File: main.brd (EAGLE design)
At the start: 50 x 95 mm, 213 parts, among them CN1 USB C 2.0, CN2 JST GH 10 Pin, CN3 15PIN 0.5MM, CN4 8 PIN FFC, CN5 NEB-21-R, CN6 S4B-XH-SM4-TB, CN7 8 PIN FFC, Q1 GSFP0449, Q2 2SCR586D, Q3 MMBT3904, SW1 DPDT, U1 TPS54302, U10 SN74LVC2G17, U11 SN74LVC2G17, U12 SN74LVC2G17, U13 SN74LVC2G17, U14 SN74LVC2G17, U15 SN74LVC2G17, U16 SN74LVC2G17, U17 SN74LVC2G17, U18 T8Q144C4, U19 SN74LVC2G17, U2 USBLC6-2SC6, U20 R2A20169SA#W5, U21 LM317MDT, U22 LM317MDT, U23 TMC2208-LA-T, U3 93LC56B-I/SN, U33 LM317MDT, U34 LM317MDT, U4 W25Q128JV, U5 TPS62065, U6 FT2232H, U7 TPS563201, U8 TCD2720BFG, U9 SN74LVC2G17

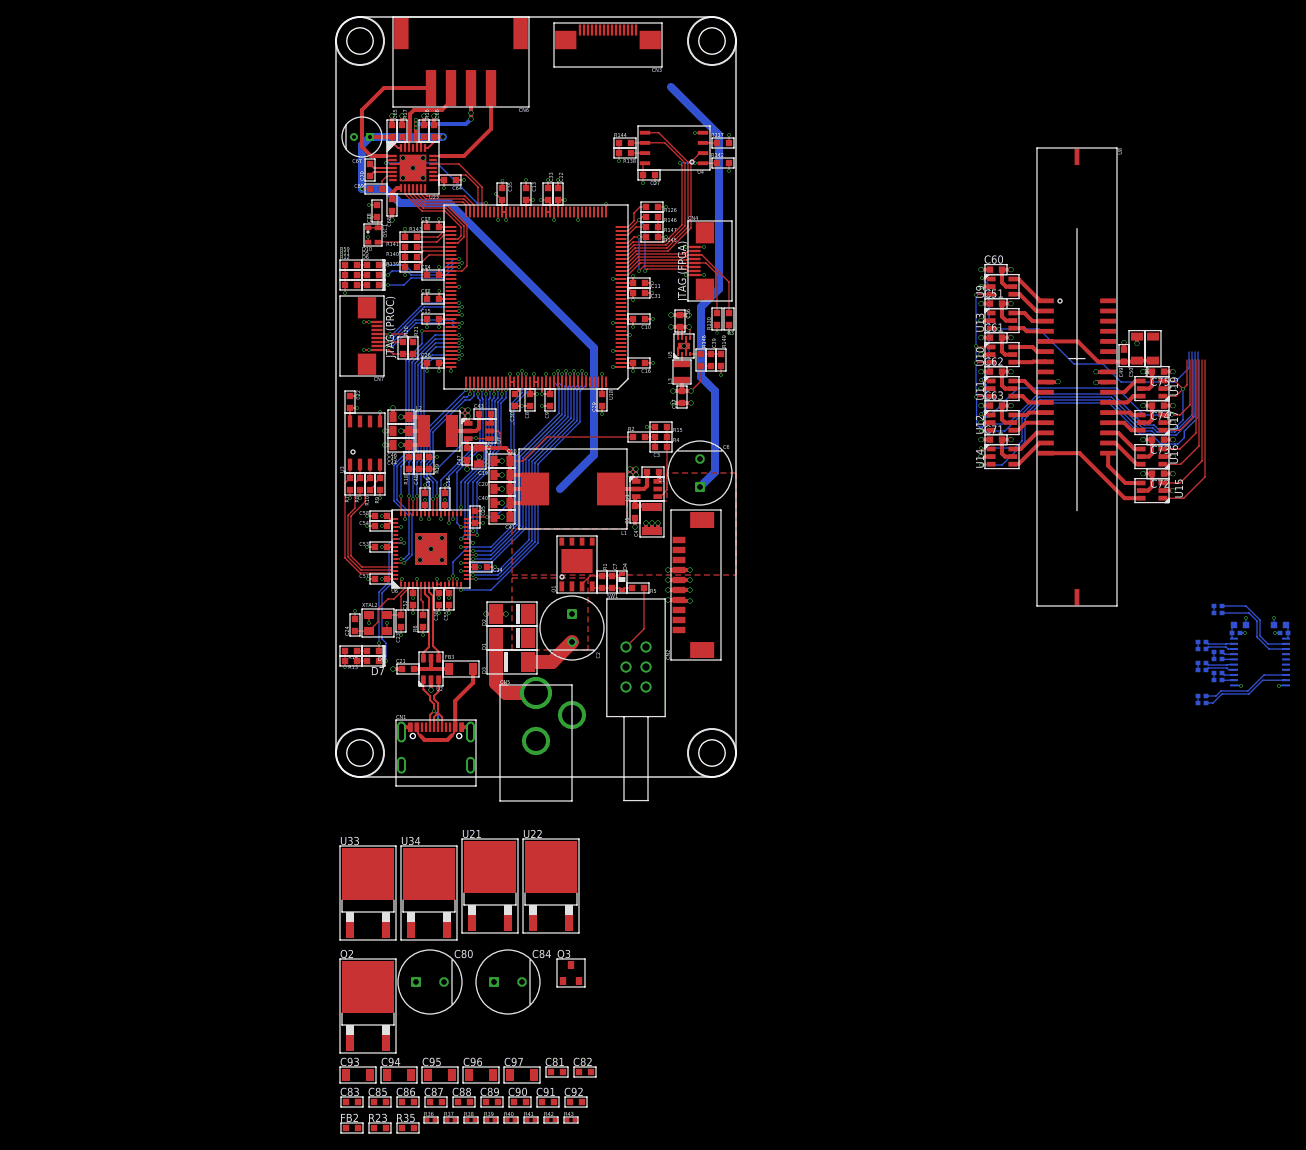
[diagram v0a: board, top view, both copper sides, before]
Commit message: FTDI and CCD routed
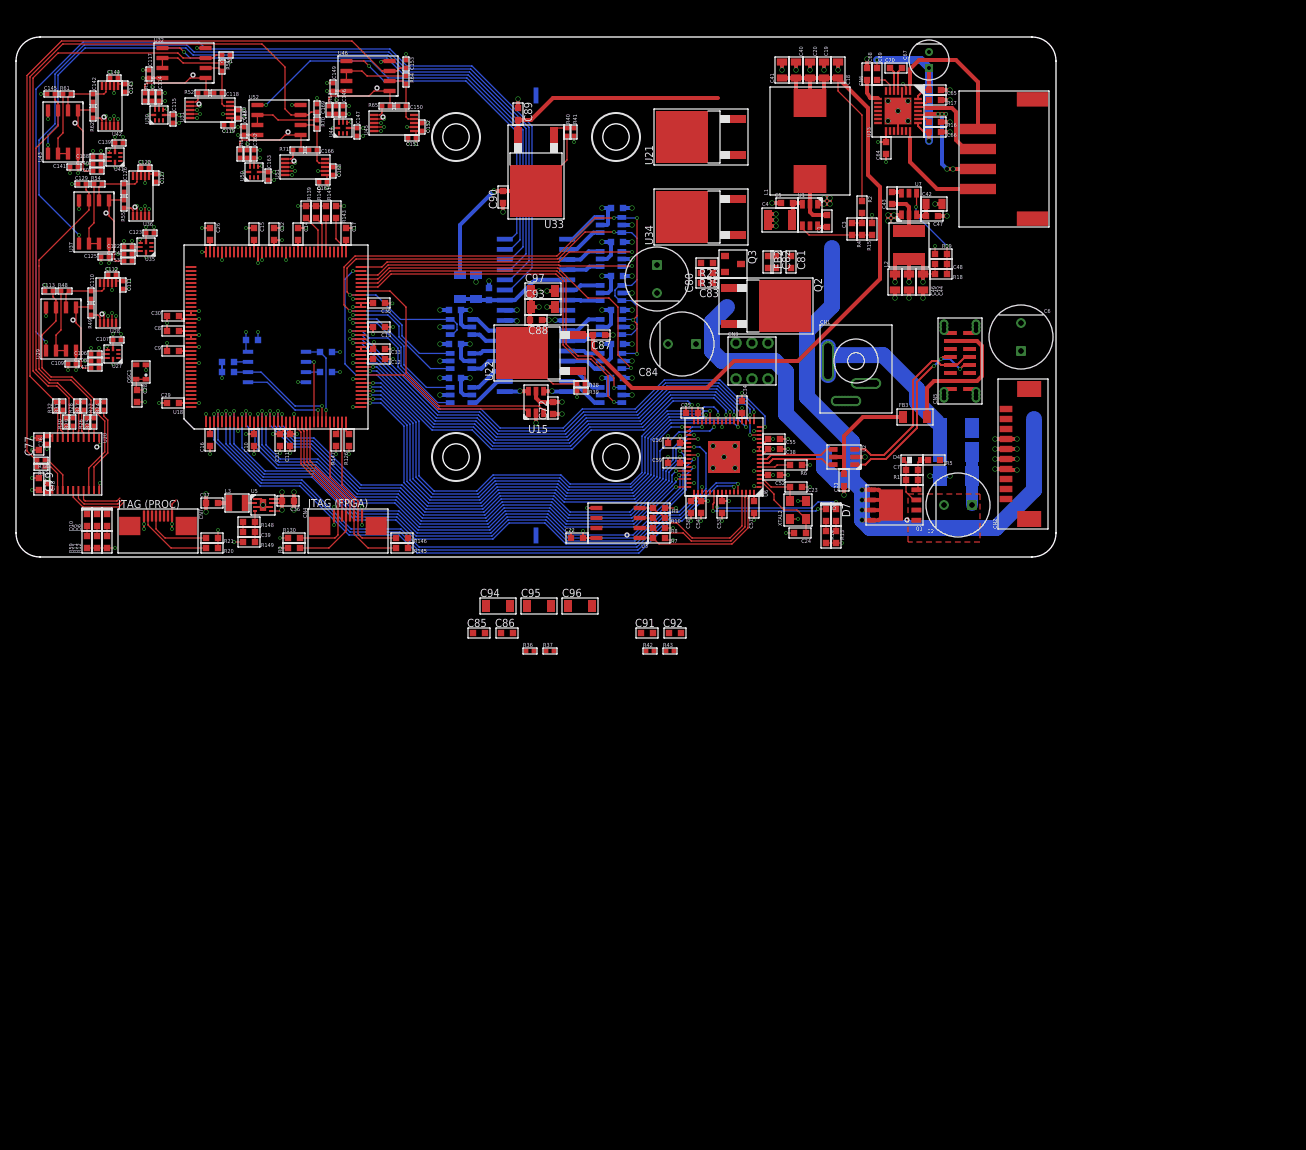
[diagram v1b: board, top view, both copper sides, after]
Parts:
- removed SW1: DPDT, ELECTROMECH:PBH2UEESNPNAGX
- added C106, C107, C109, C111, C112, C113, C114, C115, C117, C119, C120, C121, C122, C123, C125, C127, C128, C129, C138, C139, C141, C143, C144, C145, C146, C147, C149, C151, C152, C153, C162, C163, C165, C167, C168, C169: 0.1uF 16V, c_0402:0402
- added C108, C116, C124, C140, C148, C164: 220pF 25V, c_0402:0402
- added C110, C118, C126, C142, C150, C166: NO FIT, c_0402:0402
- added R47, R50, R53, R60, R63, R69: 100R, r_0402:0402
- added R48, R51, R54, R61, R64, R70: 330R, r_0402:0402
- added R49, R52, R55, R62, R65, R71: 680R, r_0402:0402
- added U27, U30, U35, U41, U44, U50: ADS7056, ICs:X2QFN8
- added U28, U31, U36, U42, U45, U51: AD5258BRMZ1-R7, ICs:MSOP10
- added U29, U32, U37, U43, U46, U52: COS8092SR, ICs:SO8
- CN1: value USB C 2.0 -> DC-012A-D010; device CONNECTORs:MC-107D -> CONNECTORs:DC-012A-D010
- CN3: value 15PIN 0.5MM -> 5.8ZSPT; device CONNECTORs:SFV15R-1STE1HLF -> ELECTROMECH:5.8ZSPT
- CN5: value NEB-21-R -> MC-118LS-H100; device CONNECTORs:NEB-21-R -> CONNECTORs:MC-118LS-H100
- R41: value 715R -> 1.69k
- R43: value 715R -> 390R
- moved C79 156.1 mm to (-62.1, -23.4), flipped to the top, turned to 270 degrees
- moved C78 155.7 mm to (-61.1, -23.9), flipped to the top, turned to 270 degrees
- moved C77 151.8 mm to (-62.1, -18.4), flipped to the top, turned to 90 degrees
- moved C76 150.6 mm to (-61.1, -17.9), flipped to the top, turned to 90 degrees
- moved U20 150.1 mm to (-57.5, -20.9), flipped to the top, turned to 270 degrees
- moved R34 148.4 mm to (-61.9, -20.4), flipped to the top, turned to 180 degrees
- moved R33 148.1 mm to (-61.9, -21.3), flipped to the top, turned to 180 degrees
- moved R30 146.9 mm to (-58.8, -15.6), flipped to the top, turned to 90 degrees
- moved R32 146.3 mm to (-60.0, -13.6), flipped to the top, turned to 90 degrees
- moved R29 146.2 mm to (-57.9, -15.6), flipped to the top, turned to 90 degrees
- moved R31 145.6 mm to (-59.1, -13.6), flipped to the top, turned to 90 degrees
- moved R26 144.8 mm to (-56.1, -15.6), flipped to the top, turned to 90 degrees
- moved R28 144.3 mm to (-57.4, -13.6), flipped to the top, turned to 90 degrees
- moved R25 144.2 mm to (-55.3, -15.6), flipped to the top, turned to 90 degrees
- moved R27 143.6 mm to (-56.5, -13.6), flipped to the top, turned to 90 degrees
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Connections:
- removed net GPIOB_N0: U18.56
- removed net GPIOB_N2: U18.59
- removed net GPIOB_N3: U18.60
- removed net GPIOB_N7: U18.65
- removed net GPIOB_P0: U18.55
- removed net GPIOB_P2: U18.58
- removed net GPIOB_P3: U18.61
- removed net GPIOB_P7: U18.66
- removed net GPIOB_TN0: U18.39
- removed net GPIOB_TN11: U18.54
- removed net GPIOB_TN2: U18.41
- removed net GPIOB_TN4: U18.43
- removed net GPIOB_TN6: U18.46
- removed net GPIOB_TN9: U18.48
- removed net GPIOB_TP0: U18.38
- removed net GPIOB_TP11: U18.53
- removed net GPIOB_TP2: U18.40
- removed net GPIOB_TP4: U18.42
- removed net GPIOB_TP6: U18.45
- removed net GPIOB_TP9: U18.47
- removed net GPIOL_12: U18.20
- removed net GPIOL_13: U18.19
- removed net GPIOL_20: U18.18
- removed net GPIOL_21: U18.17
- removed net GPIOL_22: U18.16
- removed net GPIOL_24: U18.15
- removed net GPIOL_25: U18.14
- removed net GPIOL_31: U18.11
- removed net GPIOL_32: U18.10
- removed net GPIOL_40: U18.8
- removed net GPIOL_41: U18.7
- removed net GPIOL_46: U18.6
- removed net GPIOL_53: U18.3
- removed net GPIOL_54: U18.4
- removed net PWR_LED_24V: C4.2, C5.2, C6.P, CN2.10, CN2.8, CN2.9, Q1.5, Q1.6, Q1.7, Q1.8, Q1.PAD, U1.3
- new net ADC_SPI_MISO_1: U27.2
- new net ADC_SPI_MISO_2: U35.2
- new net ADC_SPI_MISO_3: U41.2
- new net ADC_SPI_MISO_4: U30.2
- new net ADC_SPI_MISO_5: U44.2
- new net ADC_SPI_MISO_6: U50.2
- new net ADC_SPI_NCS: U27.1, U30.1, U35.1, U41.1, U44.1, U50.1
- new net ADC_SPI_SCLK: U27.3, U30.3, U35.3, U41.3, U44.3, U50.3
- new net N$100: R70.1, U52.6, U52.7
- new net N$61: C108.2, R47.2, U27.7
- new net N$62: C110.2, R47.1, R49.2, U29.1
- new net N$63: C110.1, R48.2, U28.9, U29.2
- new net N$64: R49.1, U28.1
- new net N$65: R48.1, U29.6, U29.7
- new net N$66: C116.2, R50.2, U30.7
- new net N$67: C118.2, R50.1, R52.2, U32.1
- new net N$68: C118.1, R51.2, U31.9, U32.2
- new net N$69: R52.1, U31.1
- new net N$70: R51.1, U32.6, U32.7
- new net N$71: C124.2, R53.2, U35.7
- new net N$72: C126.2, R53.1, R55.2, U37.1
- new net N$73: C126.1, R54.2, U36.9, U37.2
- new net N$74: R55.1, U36.1
- new net N$75: R54.1, U37.6, U37.7
- new net N$81: C140.2, R60.2, U41.7
- new net N$82: C142.2, R60.1, R62.2, U43.1
- new net N$83: C142.1, R61.2, U42.9, U43.2
- new net N$84: R62.1, U42.1
- new net N$85: R61.1, U43.6, U43.7
- new net N$86: C148.2, R63.2, U44.7
- new net N$87: C150.2, R63.1, R65.2, U46.1
- new net N$88: C150.1, R64.2, U45.9, U46.2
- new net N$89: R65.1, U45.1
- new net N$90: R64.1, U46.6, U46.7
- new net N$96: C164.2, R69.2, U50.7
- new net N$97: C166.2, R69.1, R71.2, U52.1
- new net N$98: C166.1, R70.2, U51.9, U52.2
- new net N$99: R71.1, U51.1
- new net POT_I2C0_SCL: U28.5, U36.5, U42.5
- new net POT_I2C0_SDA: U28.4, U36.4, U42.4
- new net POT_I2C1_SCL: U31.5, U45.5, U51.5
- new net POT_I2C1_SDA: U31.4, U45.4, U51.4
- net CCD_SH_M1: now also U15.4; no longer U15.6
- net CCD_SH_M2: now also U15.6; no longer U15.4
- net CCD_SIG_1A: now also U18.61
- net CCD_SIG_2A: now also U18.65
- net CCD_SIG_CP: now also U18.72
- net CCD_SIG_RS: now also U18.70
- net CCD_SIG_SH_M1: now also U15.3, U18.66; no longer U15.1
- net CCD_SIG_SH_M2: now also U15.1, U18.45; no longer U15.3
- net CCD_SIG_SH_S1: now also U18.67
- net CCD_SIG_SH_S2: now also U18.58
- net CCD_SIG_SH_S3: now also U18.68
- net CCD_SIG_SH_S4: now also U18.59
- net CCD_SIG_SW: now also U18.60
- net CCD_SIG_TG: now also U18.69
- net FPGA_CONF_CSI: now also CN4.3; no longer CN4.6
- net FPGA_CONF_NCRST: now also CN4.2; no longer CN4.7
- net FPGA_JTAG_TCK: now also CN4.5; no longer CN4.3
- net FPGA_JTAG_TDI: now also CN4.4; no longer CN4.2
- net FPGA_JTAG_TDO: now also CN4.7; no longer CN4.5
- net FPGA_JTAG_TMS: now also CN4.6; no longer CN4.4
- net FPGA_STATUS: no longer U18.83
- net FT_CLKOUT: now also U18.71; no longer U18.123
- net FT_CONT_NCTS: now also U18.10; no longer U18.109
- net FT_CONT_NDCD: now also U18.11; no longer U18.103
- net FT_CONT_NDSR: now also U18.16; no longer U18.105
- net FT_CONT_NDTR: now also U18.8; no longer U18.106
- net FT_CONT_NRI: now also U18.15; no longer U18.102
- net FT_CONT_NRTS: now also U18.7; no longer U18.110
- net FT_CONT_PWRSAV: now also U18.3; no longer U18.99
- net FT_CONT_RX: now also U18.17; no longer U18.111
- net FT_CONT_TX: now also U18.6; no longer U18.112
- net FT_CONT_TXDEN: now also U18.14; no longer U18.101
- net FT_D0: now also U18.56; no longer U18.139
- net FT_D1: now also U18.55; no longer U18.138
- net FT_D2: now also U18.54; no longer U18.137
- net FT_D3: now also U18.40; no longer U18.136
- net FT_D4: now also U18.39; no longer U18.135
- net FT_D5: now also U18.48; no longer U18.134
- net FT_D6: now also U18.47; no longer U18.132
- net FT_D7: now also U18.46; no longer U18.131
- net FT_NOE: now also U18.38; no longer U18.115
- net FT_NPWREN: now also U18.4; no longer U18.100
- net FT_NRD: now also U18.42; no longer U18.119
- net FT_NRST: now also U18.53; no longer U18.124
- net FT_NRXF: now also U18.43; no longer U18.117
- net FT_NSIWU: now also U18.20; no longer U18.114
- net FT_NSUSPEND: now also U18.18; no longer U18.113
- net FT_NTXE: now also U18.19; no longer U18.116
- net FT_NWR: now also U18.41; no longer U18.118
- net GND: now also C106.1, C107.1, C108.1, C109.1, C111.1, C112.1, C113.1, C114.1, C115.1, C116.1, C117.1, C119.1, C120.1, C121.1, C122.1, C123.1, C124.1, C125.1, C127.1, C128.1, C129.1, C138.1, C139.1, C140.1, C141.1, C143.1, C144.1, C145.1, C146.1, C147.1, C148.1, C149.1, C151.1, C152.1, C153.1, C162.1, C163.1, C164.1, C165.1, C167.1, C168.1, C169.1, CN1.-1, CN1.-2, CN1.-3, CN1.-4, CN1.-5, CN1.-6, CN1.-7, CN1.-8, CN3.2, CN5.A1, CN5.A12, CN5.B1, CN5.B12, CN5.SHELL1, CN5.SHELL10, CN5.SHELL11, CN5.SHELL12, CN5.SHELL2, CN5.SHELL3, CN5.SHELL4, CN5.SHELL5, CN5.SHELL6, CN5.SHELL7, CN5.SHELL8, CN5.SHELL9, U27.5, U27.8, U28.2, U28.3, U28.7, U29.4, U30.5, U30.8, U31.2, U31.3, U31.7, U32.4, U35.5, U35.8, U36.3, U36.7, U37.4, U41.5, U41.8, U42.2, U42.7, U43.4, U44.5, U44.8, U45.3, U45.7, U46.4, U50.5, U50.8, U51.2, U51.7, U52.4; no longer CN1.A12B1, CN1.B12A1, CN1.P$1, CN1.P$10, CN1.P$11, CN1.P$12, CN1.P$13, CN1.P$14, CN1.P$15, CN1.P$16, CN1.P$17, CN1.P$18, CN1.P$19, CN1.P$2, CN1.P$20, CN1.P$21, CN1.P$22, CN1.P$23, CN1.P$24, CN1.P$3, CN1.P$4, CN1.P$5, CN1.P$6, CN1.P$7, CN1.P$8, CN1.P$9, CN5.3, SW1.2
- net N$11: now also CN3.3; no longer SW1.3
- net N$12: now also CN5.A6, CN5.B6; no longer CN1.A6, CN1.B6
- net N$13: now also CN5.A7, CN5.B7; no longer CN1.A7, CN1.B7
- net N$41: now also CN5.A4, CN5.A9, CN5.B4, CN5.B9; no longer CN1.A9B4, CN1.B9A4
- net N$5: now also CN1.+1, CN1.+10, CN1.+11, CN1.+2, CN1.+3, CN1.+4, CN1.+5, CN1.+6, CN1.+7, CN1.+8, CN1.+9; no longer CN5.1
- net PROC_JTAG_TCK: now also CN7.5, R21.1; no longer CN7.3, R20.1, U18.97
- net PROC_JTAG_TDI: now also CN7.4; no longer CN7.2, U18.98
- net PROC_JTAG_TDO: now also CN7.7, R20.1; no longer CN7.5, R21.1, U18.92
- net PROC_JTAG_TMS: now also CN7.6; no longer CN7.4, U18.93
- net PROC_SCANNING: no longer U18.81
- net PROC_STATUS: no longer U18.82
- net PWR_ANA_3V3: now also C106.2, C114.2, C122.2, C138.2, C146.2, C162.2, U27.6, U30.6, U35.6, U41.6, U44.6, U50.6
- net PWR_ANA_5V: now also C109.2, C112.2, C117.2, C120.2, C125.2, C128.2, C141.2, C144.2, C149.2, C152.2, C165.2, C168.2, U28.8, U29.8, U31.8, U32.8, U36.8, U37.8, U42.8, U43.8, U45.8, U46.8, U51.8, U52.8
- net PWR_BUS_24V_UNREG: now also C4.2, C5.2, C6.P, CN2.10, CN2.8, CN2.9, Q1.5, Q1.6, Q1.7, Q1.8, Q1.PAD, U1.3
- net PWR_SYS_3V3: now also C107.2, C111.2, C115.2, C119.2, C123.2, C127.2, C139.2, C143.2, C147.2, C151.2, C163.2, C167.2, U27.4, U28.6, U30.4, U31.6, U35.4, U36.2, U36.6, U41.4, U42.3, U42.6, U44.4, U45.2, U45.6, U50.4, U51.3, U51.6
- net SEN_OFFSET_OS1: now also C113.2, U29.3
- net SEN_OFFSET_OS2: now also C129.2, U37.3
- net SEN_OFFSET_OS3: now also C145.2, U43.3
- net SEN_OFFSET_OS4: now also C121.2, U32.3
- net SEN_OFFSET_OS5: now also C153.2, R33.2, R34.2, U46.3; no longer R31.2, R32.2
- net SEN_OFFSET_OS6: now also C169.2, R31.2, R32.2, U52.3; no longer R33.2, R34.2
- net SEN_SIG_OS1: now also U29.5
- net SEN_SIG_OS2: now also U37.5
- net SEN_SIG_OS3: now also U43.5
- net SEN_SIG_OS4: now also U32.5
- net SEN_SIG_OS5: now also U46.5
- net SEN_SIG_OS6: now also U52.5
- net STP_CLK: no longer U18.71
- net STP_DIA: no longer U18.84
- net STP_DIR: no longer U18.68
- net STP_IDX: no longer U18.72
- net STP_MS1: no longer U18.76
- net STP_MS2: no longer U18.77
- net STP_NEN: no longer U18.67
- net STP_STP: no longer U18.69
- net STP_UART_IO: no longer U18.70
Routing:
- net PWR_BUS_24V_UNREG: track 0.00 -> 127.0 mm, vias 0 -> 4
- net SEN_SIG_OS1: track 0.70 -> 125.0 mm, vias 0 -> 1
- net PWR_FPGA_1V2: track 145.9 -> 21.9 mm, vias 13 -> 3
- net SEN_SIG_OS2: track 0.75 -> 110.6 mm, vias 0 -> 1
- net SEN_OFFSET_OS5: track 0.88 -> 100.4 mm
- net SEN_SIG_OS3: track 0.62 -> 94.2 mm, vias 0 -> 1
- net SEN_OFFSET_OS6: track 0.88 -> 87.3 mm
- net SEN_OFFSET_OS4: track 0.88 -> 71.2 mm
- net SEN_SIG_OS4: track 0.00 -> 66.9 mm, vias 0 -> 1
- net FT_CONT_TX: track 19.9 -> 80.8 mm
- net GND: track 170.8 -> 231.4 mm, vias 155 -> 237
- net FT_CONT_NRTS: track 19.2 -> 78.6 mm
- net PWR_LED_24V: track 58.3 -> 0.00 mm
- net SEN_SIG_OS6: track 0.00 -> 54.7 mm, vias 0 -> 1
- net FT_CONT_NCTS: track 20.2 -> 74.2 mm
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- added copper zone on layer 3, net PWR_CLK_5V
- removed copper zone on layer 1, net PWR_LED_24V
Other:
- board size 50 x 95 mm -> 130 x 65 mm

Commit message: Board routed, needs motor driver and thorough review
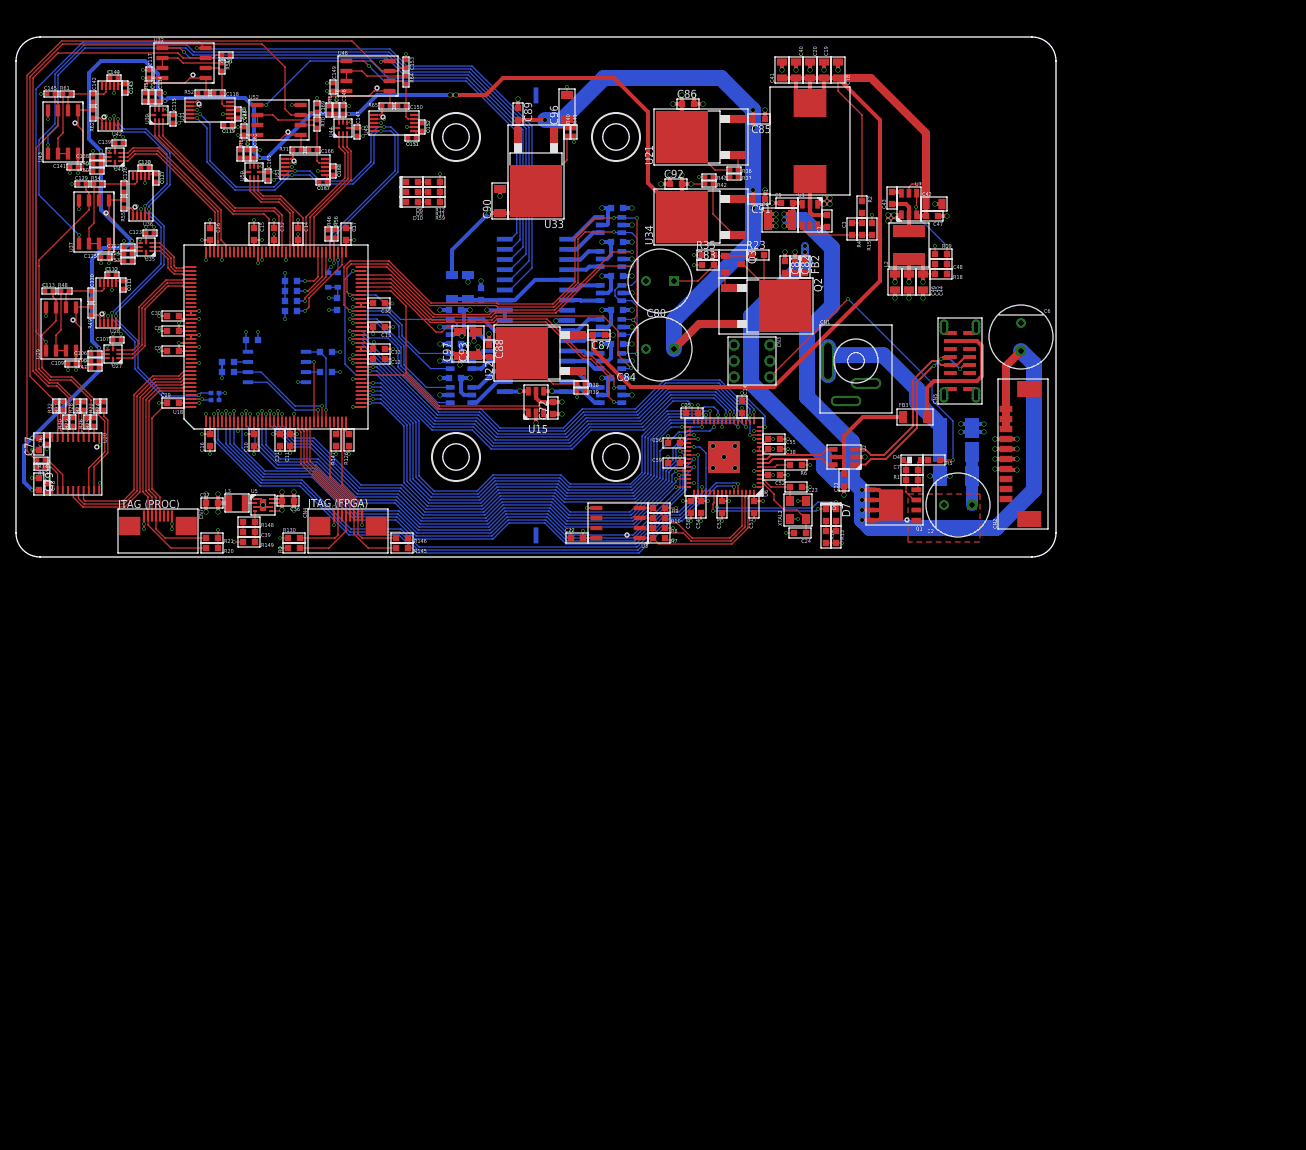
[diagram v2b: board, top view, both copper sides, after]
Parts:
- removed C64, C65, C66, C69: 100nF 16V, CAPACITORS:0603
- removed C67: 100uF 25V, CAPACITORS:5MM_RADIAL_2MM_PITCH
- removed C68: 2.2uF 10V, c_0603:0603
- removed C70: 0.022uF 50V, c_0603:0603
- removed C94, C95: 10uF 10V, c_1206:1206
- removed CN6: S4B-XH-SM4-TB, CONNECTORs:S4B-XH-SM4-TB
- removed R16, R17: 0.33R, RESISTORS:0603
- removed U23: TMC2208-LA-T, ICs:QFN28
- added R44, R45, R46, R56: 2.2k, r_0402:0402
- C90: value 1uF 10V -> 1uF 16V; device c_0603:0603 -> c_1206:1206
- moved C85 73.2 mm to (27.9, 22.2), turned to 180 degrees
- moved C86 69.9 mm to (19.0, 24.1), turned to 180 degrees
- moved R36 65.3 mm to (24.8, 15.9), turned to 180 degrees
- moved R37 63.6 mm to (24.8, 15.0)
- moved C96 62.4 mm to (3.88, 23.8), turned to 90 degrees
- moved R12 60.8 mm to (-12.8, 14.4), turned to 0 degrees
- moved R11 60.7 mm to (-12.8, 13.1), turned to 0 degrees
- moved R59 60.7 mm to (-12.8, 11.9), turned to 0 degrees
- moved R43 59.5 mm to (21.6, 15.0)
- moved R42 58.8 mm to (21.6, 14.1), turned to 180 degrees
- moved D6 56.9 mm to (-15.5, 14.4), turned to 0 degrees
- moved D5 56.8 mm to (-15.5, 13.1), turned to 0 degrees
- moved D10 56.8 mm to (-15.5, 11.9), turned to 0 degrees
- moved C92 56.1 mm to (17.5, 14.1)
- moved C91 56.0 mm to (27.9, 12.2), turned to 180 degrees
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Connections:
- removed net ADC_SPI_NCS: U27.1, U30.1, U35.1, U41.1, U44.1, U50.1
- removed net ADC_SPI_SCLK: U27.3, U30.3, U35.3, U41.3, U44.3, U50.3
- removed net GPIOL_64: U18.144
- removed net GPIOL_65: U18.141
- removed net GPIOL_66: U18.142
- removed net GPIOL_67: U18.140
- removed net GPIOR_128: U18.90
- removed net GPIOR_129: U18.89
- removed net GPIOR_132: U18.87
- removed net GPIOR_133: U18.86
- removed net N$18: C68.2, U23.8
- removed net N$24: C69.1, U23.6
- removed net N$37: C70.2, U23.5
- removed net N$38: C70.1, U23.4
- removed net N$47: R16.1, U23.23
- removed net N$48: R17.1, U23.27
- removed net STP_CLK: U23.13
- removed net STP_DIA: U23.11
- removed net STP_DIR: U23.19
- removed net STP_IDX: U23.12
- removed net STP_MS1: U23.9
- removed net STP_MS2: U23.10
- removed net STP_MTR_A1: CN6.2, U23.24
- removed net STP_MTR_A2: CN6.1, U23.21
- removed net STP_MTR_B1: CN6.3, U23.26
- removed net STP_MTR_B2: CN6.4, U23.1
- removed net STP_NEN: U23.2
- removed net STP_STP: U23.16
- removed net STP_UART_IO: U23.14
- new net ADC_SPI_NCS_1: U18.114, U27.1
- new net ADC_SPI_NCS_2: U18.111, U35.1
- new net ADC_SPI_NCS_3: U18.106, U41.1
- new net ADC_SPI_NCS_4: U18.92, U30.1
- new net ADC_SPI_NCS_5: U18.83, U44.1
- new net ADC_SPI_NCS_6: U18.87, U50.1
- new net ADC_SPI_SCLK_1: U18.112, U27.3
- new net ADC_SPI_SCLK_2: U18.109, U35.3
- new net ADC_SPI_SCLK_3: U18.103, U41.3
- new net ADC_SPI_SCLK_4: U18.89, U30.3
- new net ADC_SPI_SCLK_5: U18.81, U44.3
- new net ADC_SPI_SCLK_6: U18.84, U50.3
- new net N$101: U18.100
- new net N$102: U18.99
- new net N$103: U18.98
- new net N$104: U18.97
- new net N$105: U18.93
- new net N$59: U18.102
- new net N$60: U18.101
- new net N$76: U18.134
- new net N$77: U18.132
- new net N$78: U18.131
- new net N$79: U18.124
- new net N$80: U18.123
- new net N$91: U18.119
- new net N$92: U18.118
- new net N$93: U18.117
- new net N$94: U18.116
- new net N$95: U18.115
- net ADC_SPI_MISO_1: now also U18.113
- net ADC_SPI_MISO_2: now also U18.110
- net ADC_SPI_MISO_3: now also U18.105
- net ADC_SPI_MISO_4: now also U18.90
- net ADC_SPI_MISO_5: now also U18.82
- net ADC_SPI_MISO_6: now also U18.86
- net DAC_SPI_MOSI: now also U18.135
- net DAC_SPI_NCS: now also U18.137
- net DAC_SPI_SCLK: now also U18.136
- net GND: no longer C64.1, C65.1, C66.1, C67.2, C68.1, C94.1, C95.1, R16.2, R17.2, U23.18, U23.29, U23.3
- net N$52: no longer C95.2
- net N$55: no longer C94.2
- net POT_I2C0_SCL: now also R44.1, U18.141
- net POT_I2C0_SDA: now also R45.1, U18.142
- net POT_I2C1_SCL: now also R46.1, U18.77
- net POT_I2C1_SDA: now also R56.1, U18.76
- net PROC_JTAG_TCK: now also U18.140
- net PROC_JTAG_TDI: now also U18.144
- net PROC_JTAG_TDO: now also U18.138
- net PROC_JTAG_TMS: now also U18.139
- net PWR_SYS_12V: no longer C65.2, C66.2, C67.1, C69.2, U23.22, U23.28
- net PWR_SYS_3V3: now also R44.2, R45.2, R46.2, R56.2; no longer C64.2, U23.15
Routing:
- net PWR_ANA_3V3: track 16.8 -> 188.8 mm, vias 8 -> 12
- net PWR_FPGA_1V2: track 21.9 -> 162.8 mm, vias 3 -> 13
- net POT_I2C1_SDA: track 3.75 -> 64.2 mm, vias 3 -> 4
- net POT_I2C1_SCL: track 2.62 -> 61.7 mm, vias 3 -> 4
- net PWR_ANA_UNREG: track 28.0 -> 85.5 mm, vias 0 -> 5
- net POT_I2C0_SDA: track 3.75 -> 57.9 mm, vias 3 -> 4
- net POT_I2C0_SCL: track 2.62 -> 55.3 mm, vias 3 -> 4
- net N$11: track 0.00 -> 41.0 mm, vias 0 -> 2
- net PWR_BUS_24V_UNREG: track 127.0 -> 165.6 mm, vias 4 -> 9
- net ADC_SPI_MISO_4: track 0.00 -> 25.6 mm
- net ADC_SPI_SCLK_4: track 0.00 -> 25.5 mm
- net ADC_SPI_NCS_4: track 0.00 -> 24.7 mm
- net DAC_SPI_MOSI: track 5.98 -> 28.4 mm
- net DAC_SPI_SCLK: track 7.00 -> 29.0 mm
- net PROC_JTAG_TDO: track 9.57 -> 31.3 mm
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- added copper zone on layer 3, net PWR_ANA_5V
